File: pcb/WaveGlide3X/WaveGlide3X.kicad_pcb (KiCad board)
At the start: 2 copper layers, 89 x 95 mm, 29 parts

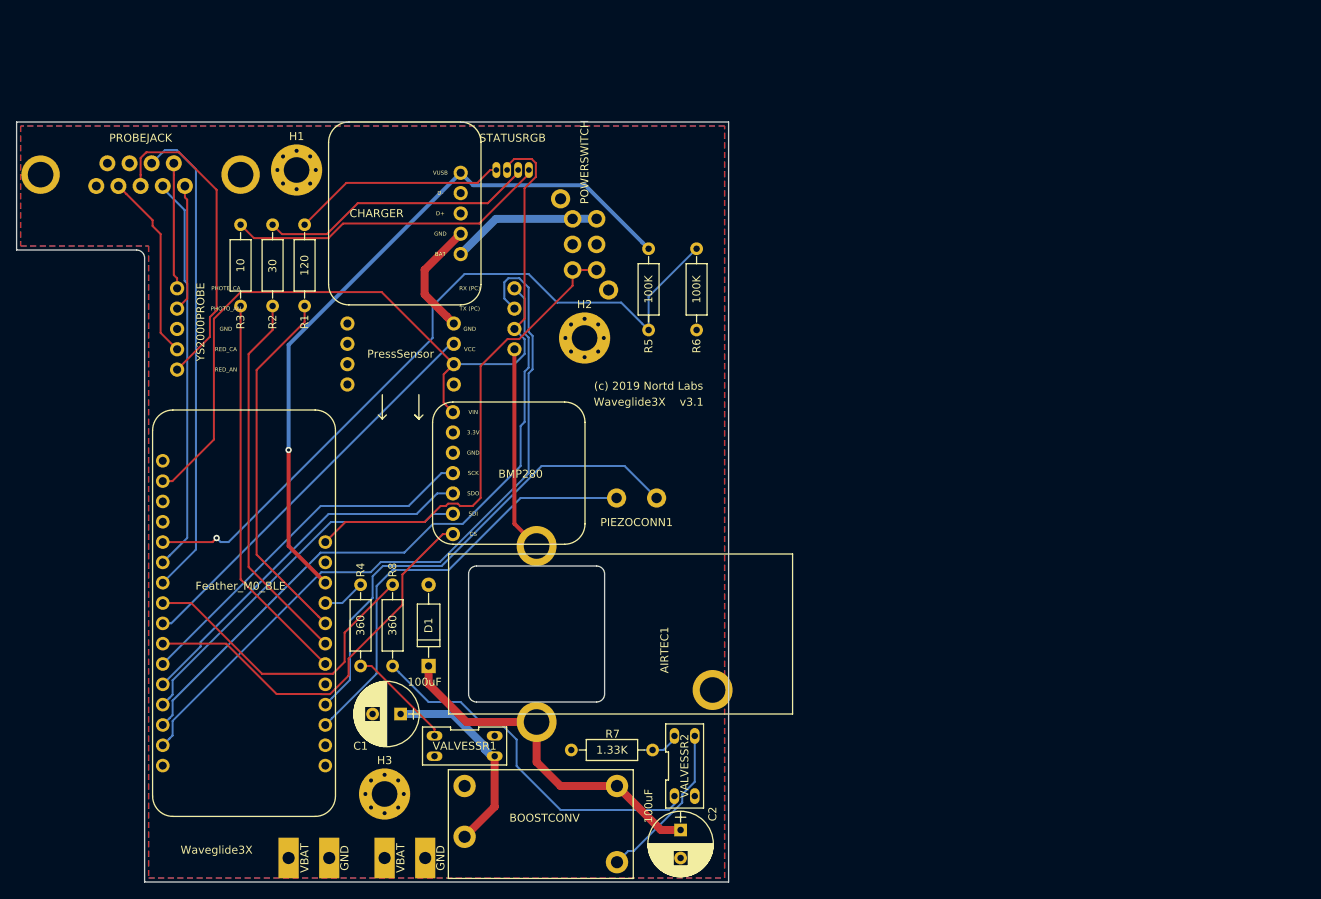
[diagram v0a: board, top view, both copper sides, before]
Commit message: as finished for 3X v3.1
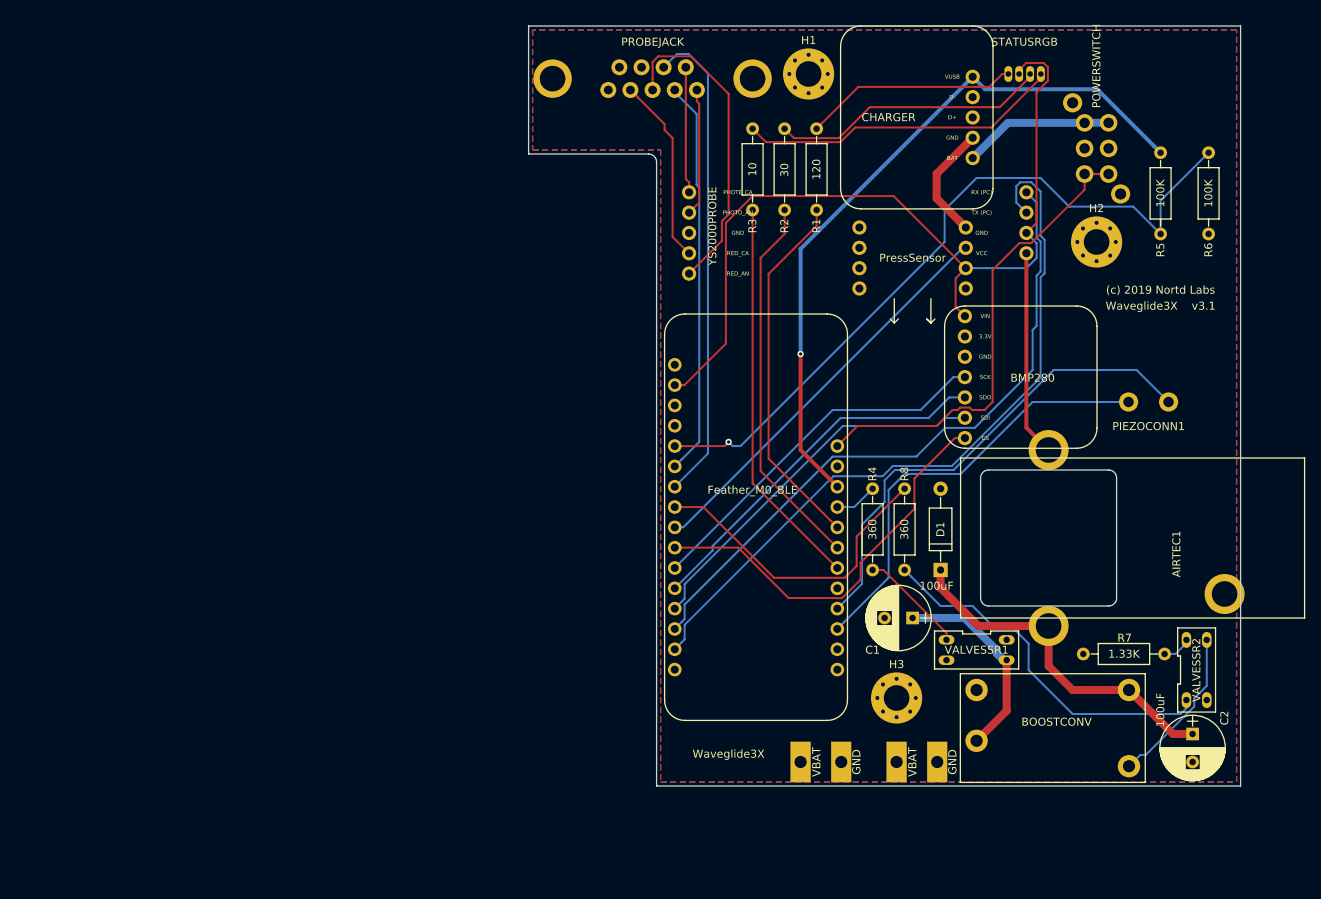
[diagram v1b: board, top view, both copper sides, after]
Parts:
- moved AIRTEC1 65.1 mm to (194.0, 122.0)
- moved BMP280 65.1 mm to (149.0, 83.0)
- moved BOOSTCONV1 65.1 mm to (153.0, 131.0)
- moved C1 65.1 mm to (145.0, 122.0)
- moved C2 65.1 mm to (180.0, 136.5)
- moved CHARGER1 65.1 mm to (136.0, 48.0)
- moved D1 65.1 mm to (148.5, 116.0)
- moved DIFFPRESSURE1 65.1 mm to (145.0, 77.0)
- moved Feather_M0_BLE1 65.1 mm to (114.0, 84.0)
- moved H1 65.1 mm to (132.0, 54.0)
- moved H2 65.1 mm to (168.0, 75.0)
- moved H3 65.1 mm to (143.0, 132.0)
- moved PIEZOCONN1 65.1 mm to (174.5, 95.0)
- moved POWERSWITCH1 65.1 mm to (171.0, 69.0)
- moved PROBEJACK1 65.1 mm to (112.5, 56.0)
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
